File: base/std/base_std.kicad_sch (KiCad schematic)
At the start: 19 parts, among them J1 Moat_Wire_12, J10 1wireConn, J2 Moat_Bus_wire, J3 I2C, J4 Conn_01x08, Q1 2N7002

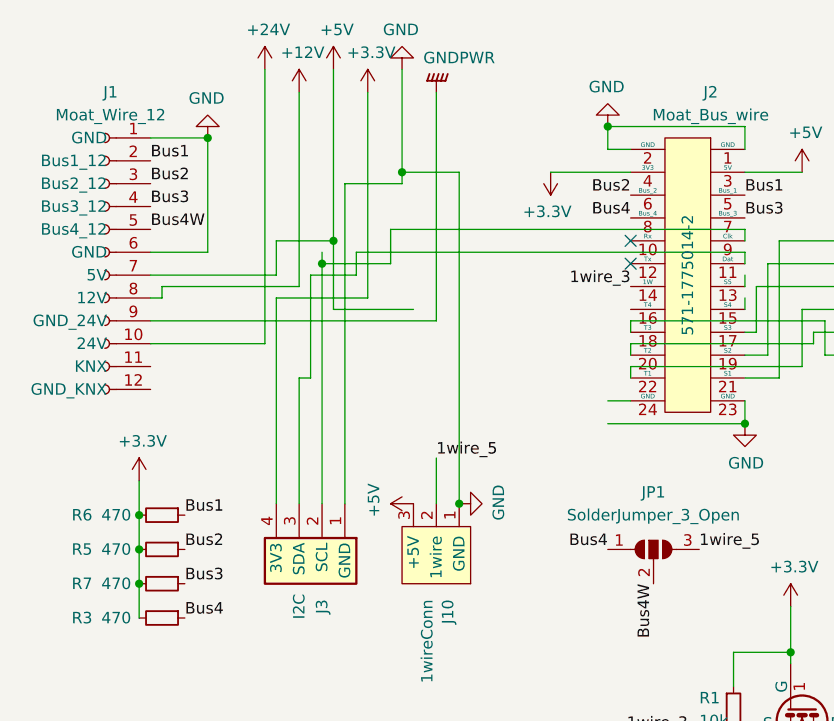
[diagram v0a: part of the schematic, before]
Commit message: misc updates I didn't bother checking in, oops
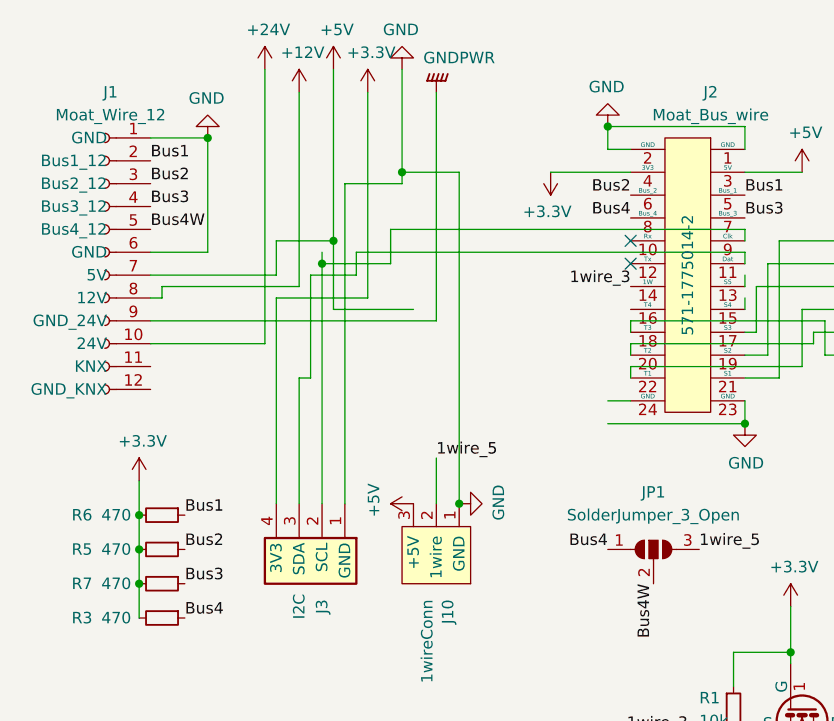
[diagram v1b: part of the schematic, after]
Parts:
- D1: symbol Diode:BAT54S -> localparts:BAT54SW
- D2, D3, D4, D5, D6: footprint Package_TO_SOT_SMD:SOT-323_SC-70 -> Package_TO_SOT_SMD:SOT-23; symbol Diode:BAT54SW -> localparts:BAT54SW
